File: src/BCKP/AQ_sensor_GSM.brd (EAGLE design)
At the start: 110 x 64 mm, 111 parts, among them J1 F-1X03-SIP-100-32, J2 53261-0871, J3 PJ-002BH, Q2 MMBT2222, Q3 MMBT2222, Q4 MMBT2222, Q5 MMBT2222, Q6 MMBT2222, Q7 MMBT2222, U3 TEXAS_INSTRUMENTS_LM1117IMP-3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, U5 TXS0108EPWR

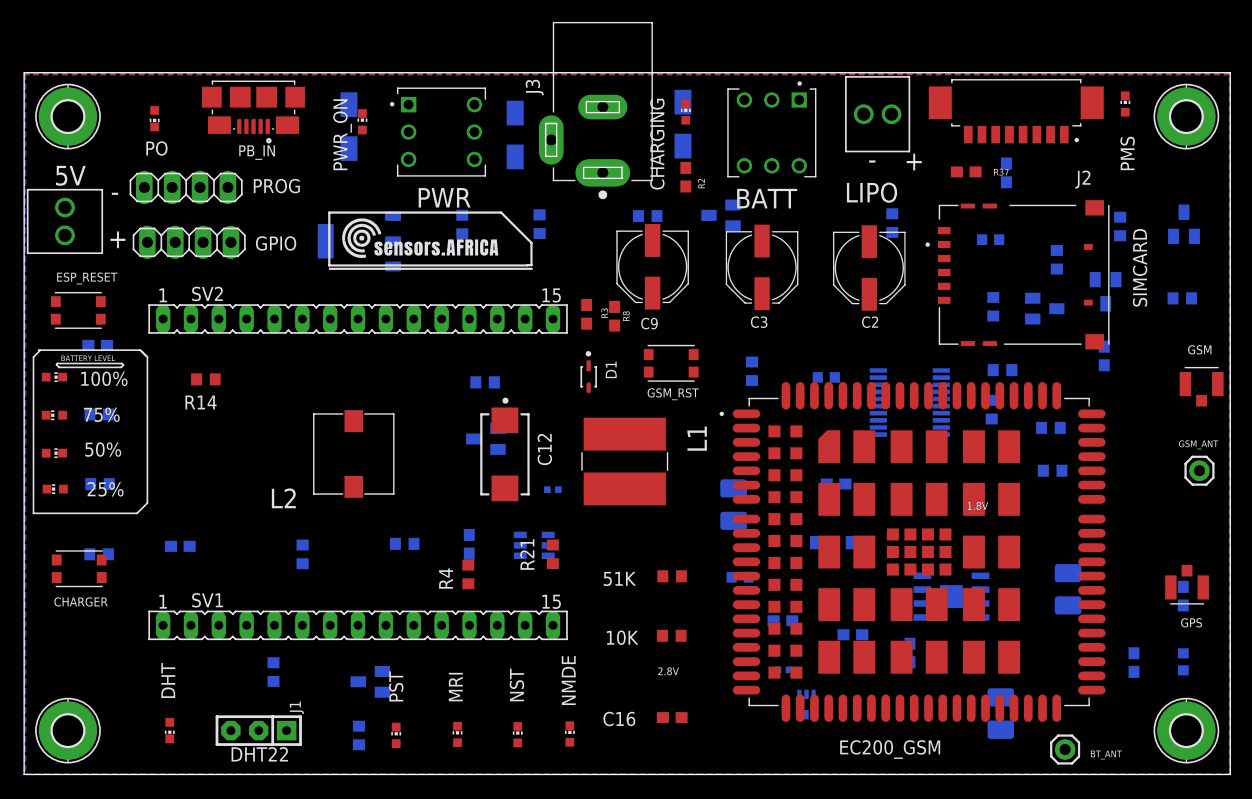
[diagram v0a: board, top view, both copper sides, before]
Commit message: JLCPCB V2
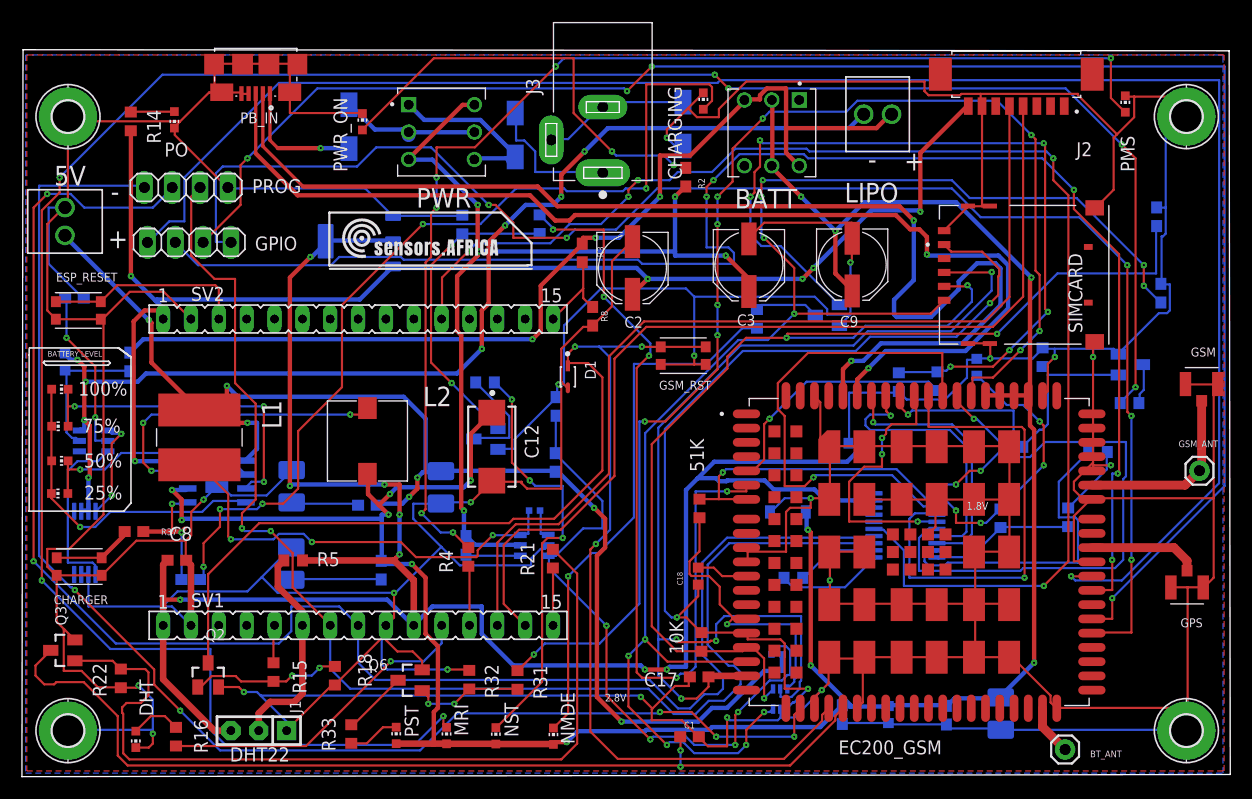
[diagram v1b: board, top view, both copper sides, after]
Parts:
- added C23: TAJB106K016RNJ, Resistor_Capacitor:CAP_TANT_B
- added C4: 100nf, 06035C104K4T2A:CAPC1608X90N
- added Q1: FS8205A, FS8205A:SOP65P640X120-8N
- added R10: 100R, SparkFun-Resistors:0603
- added R17: 2R, SparkFun-Resistors:0603
- added R9: 1k, SparkFun-Resistors:0603
- added U1: DW01-P, DW01-P:SOT23-6L
- SV1, SV2: value (none) -> ZX-PM2.54-1-15PY
- moved Q3 100.6 mm to (3.79, 11.0), flipped to the top, turned to 90 degrees
- moved R22 100.0 mm to (9.08, 8.44), flipped to the top, turned to 90 degrees
- moved Q2 98.0 mm to (17.0, 8.75), flipped to the top
- moved R18 84.6 mm to (28.6, 8.69), flipped to the top, turned to 90 degrees
- moved R37 82.7 mm to (10.3, 21.8)
- moved U$2 67.8 mm to (17.8, 26.4)
- moved R20 66.0 mm to (15.5, 17.5), turned to 0 degrees
- moved R29 65.0 mm to (70.4, 17.6)
- moved C17 62.6 mm to (61.8, 8.58), flipped to the top, turned to 180 degrees
- moved C16 59.0 mm to (103.9, 43.6), flipped to the bottom, turned to 90 degrees
- moved C30 58.0 mm to (38.3, 25.9)
- moved C1 51.4 mm to (60.9, 3.12), flipped to the top, turned to 0 degrees
- moved R19 42.2 mm to (32.8, 18.3), turned to 90 degrees
- moved C24 40.7 mm to (24.6, 18.9), turned to 90 degrees
- moved R31 39.8 mm to (45.3, 8.30), flipped to the top, turned to 270 degrees
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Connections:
- new net BATT-: C4.2, LIPO.2, Q1.2, Q1.3, U1.6
- new net N$13: C23.1, R17.1
- new net N$19: Q1.5, U1.3
- new net N$37: C4.1, R10.1, U1.5
- new net N$47: R9.1, U1.2
- new net N$9: Q1.4, U1.1
- net 5V_IN: now also R17.2
- net GND: now also C23.2, Q1.6, Q1.7, R9.2; no longer LIPO.2
- net LBV: now also R10.2
- net USIM_VDD: now also SIMCARD.C1
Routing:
- net GND: track 0.00 -> 936.4 mm, vias 0 -> 20
- net V_LIPO: track 0.00 -> 231.7 mm, vias 0 -> 13
- net N$44: track 0.00 -> 214.9 mm, vias 0 -> 7
- net +3V3: track 0.00 -> 185.8 mm, vias 0 -> 8
- net G_ADC0: track 0.00 -> 162.2 mm, vias 0 -> 1
- net G_I2C_SDA: track 0.00 -> 158.6 mm, vias 0 -> 4
- net MCU_RXD: track 0.00 -> 151.0 mm, vias 0 -> 2
- net SIMCLK: track 0.00 -> 141.2 mm, vias 0 -> 11
- net G_ADC1: track 0.00 -> 138.3 mm, vias 0 -> 5
- net G_I2C_SCL: track 0.00 -> 138.0 mm, vias 0 -> 5
- net GSM_RST: track 0.00 -> 135.4 mm, vias 0 -> 3
- net 5V_OUT: track 0.00 -> 127.6 mm, vias 0 -> 6
- net G_USB_BOOT: track 0.00 -> 125.6 mm, vias 0 -> 5
- net MCU_DTR: track 0.00 -> 125.2 mm, vias 0 -> 5
- net 5V_IN: track 0.00 -> 123.8 mm, vias 0 -> 7
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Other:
- board size 110 x 64 mm -> 110.2 x 66.3 mm
